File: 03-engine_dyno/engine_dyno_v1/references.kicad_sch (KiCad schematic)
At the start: 5 parts, among them U5 AD5689RBRUZ

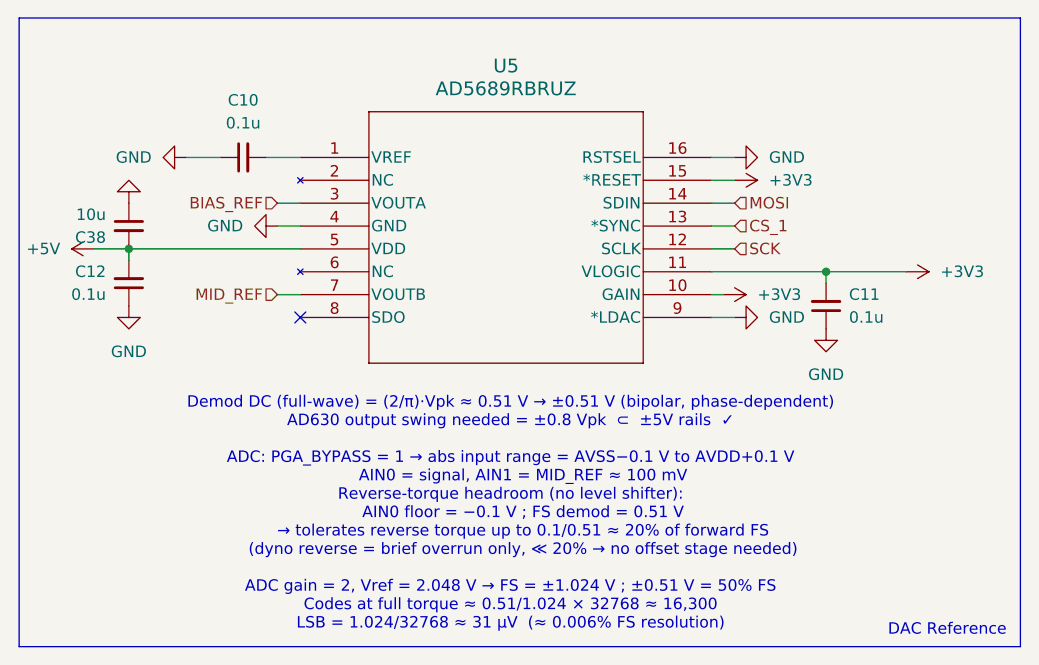
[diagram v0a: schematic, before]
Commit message: polished
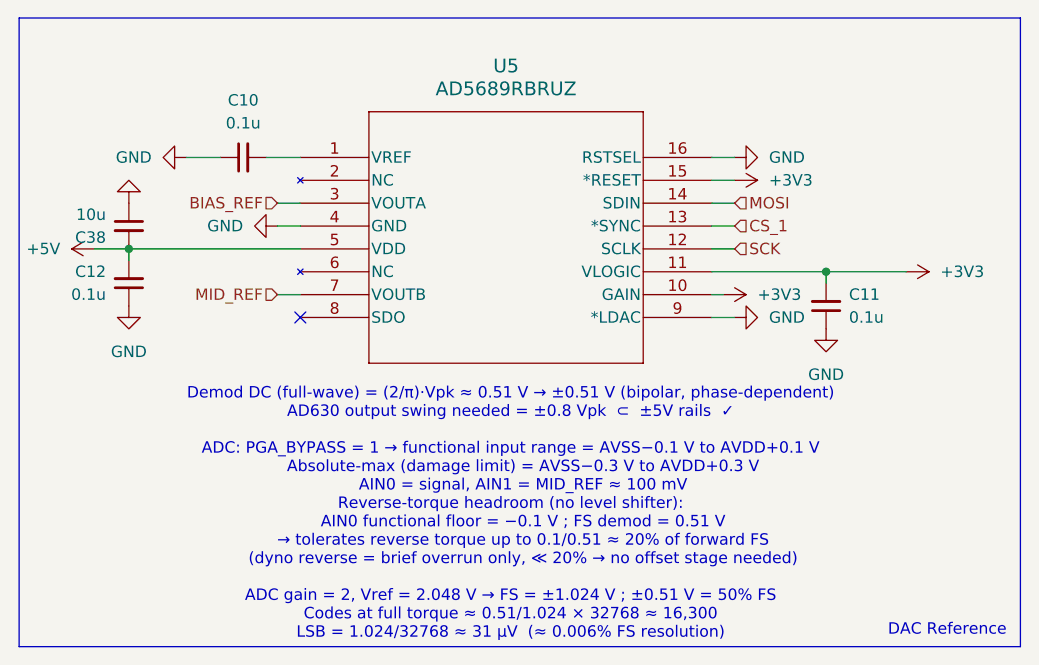
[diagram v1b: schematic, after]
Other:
- note added: "Demod DC (full-wave) = (2/π)·Vpk ≈ 0.51 V → ±0.51 V (bipolar, phase-dependent) AD630 output swing needed = ±0.8 Vpk ⊂ ±5V rails ✓ ADC: PGA_BYPASS = 1 → functional input range = AVSS−0.1 V to AVDD+0.1 V Absolute-max (damage limit) = AVSS−0.3 V to AVDD+0.3 V AIN0 = signal, AIN1 = MID_REF ≈ 100 mV Reverse-torque headroom (no level shifter): AIN0 functional floor = −0.1 V ; FS demod = 0.51 V → tolera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"
- note removed: "Demod DC (full-wave) = (2/π)·Vpk ≈ 0.51 V → ±0.51 V (bipolar, phase-dependent) AD630 output swing needed = ±0.8 Vpk ⊂ ±5V rails ✓ ADC: PGA_BYPASS = 1 → abs input range = AVSS−0.1 V to AVDD+0.1 V AIN0 = signal, AIN1 = MID_REF ≈ 100 mV Reverse-torque headroom (no level shifter): AIN0 floor = −0.1 V ; FS demod = 0.51 V → tolerates reverse torque up to 0.1/0.51 ≈ 20% of forward FS (dyno reverse = bri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"
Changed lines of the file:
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@@
 		)
 	)
-	(text "Demod DC (full-wave) = (2/π)·Vpk ≈ 0.51 V → ±0.51 V (bipolar, phase-dependent)\nAD630 output swing needed = ±0.8 Vpk  ⊂  ±5V rails  ✓\n\nADC: PGA_BYPASS = 1 → abs input range = AVSS−0.1 V to AVDD+0.1 V\n     AIN0 = signal, AIN1 = MID_REF ≈ 100 mV\nReverse-torque headroom (no level shifter):\n     AIN0 floor = −0.1 V ; FS demod = 0.51 V\n     → tolerates reverse torque up to 0.1/0.51 ≈ 20% of forward FS\n     (dyno reverse = brief overrun only, ≪ 20% → no offset stage needed)\n\nADC gain = 2, Vref = 2.048 V → FS = ±1.024 V ; ±0.51 V = 50% FS\nCodes at full torque ≈ 0.51/1.024 × 32768 ≈ 16,300\nLSB = 1.024/32768 ≈ 31 µV  (≈ 0.006% FS resolution)"
+	(text "Demod DC (full-wave) = (2/π)·Vpk ≈ 0.51 V → ±0.51 V (bipolar, phase-dependent)\nAD630 output swing needed = ±0.8 Vpk  ⊂  ±5V rails  ✓\n\nADC: PGA_BYPASS = 1 → functional input range = AVSS−0.1 V to AVDD+0.1 V\n     Absolute-max (damage limit) = AVSS−0.3 V to AVDD+0.3 V\n     AIN0 = signal, AIN1 = MID_REF ≈ 100 mV\nReverse-torque headroom (no level shifter):\n     AIN0 functional floor = −0.1 V ; FS demod = 0.51 V\n     → tolerates reverse torque up to 0.1/0.51 ≈ 20% of forward FS\n     (dyno reverse = brief overrun only, ≪ 20% → no offset stage needed)\n\nADC gain = 2, Vref = 2.048 V → FS = ±1.024 V ; ±0.51 V = 50% FS\nCodes at full torque ≈ 0.51/1.024 × 32768 ≈ 16,300\nLSB = 1.024/32768 ≈ 31 µV  (≈ 0.006% FS resolution)"
 		(exclude_from_sim no)
 		(at 150.368 132.334 0)
